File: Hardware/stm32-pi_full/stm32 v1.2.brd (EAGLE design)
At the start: 131.4 x 105.8 mm, 288 parts, among them J1 JUMPER-SMT_2_NC_TRACE_NO-SILK, Q1 PNP, Q2 NPN, Q3 NPN, U1 ESP32-WROOM-32D

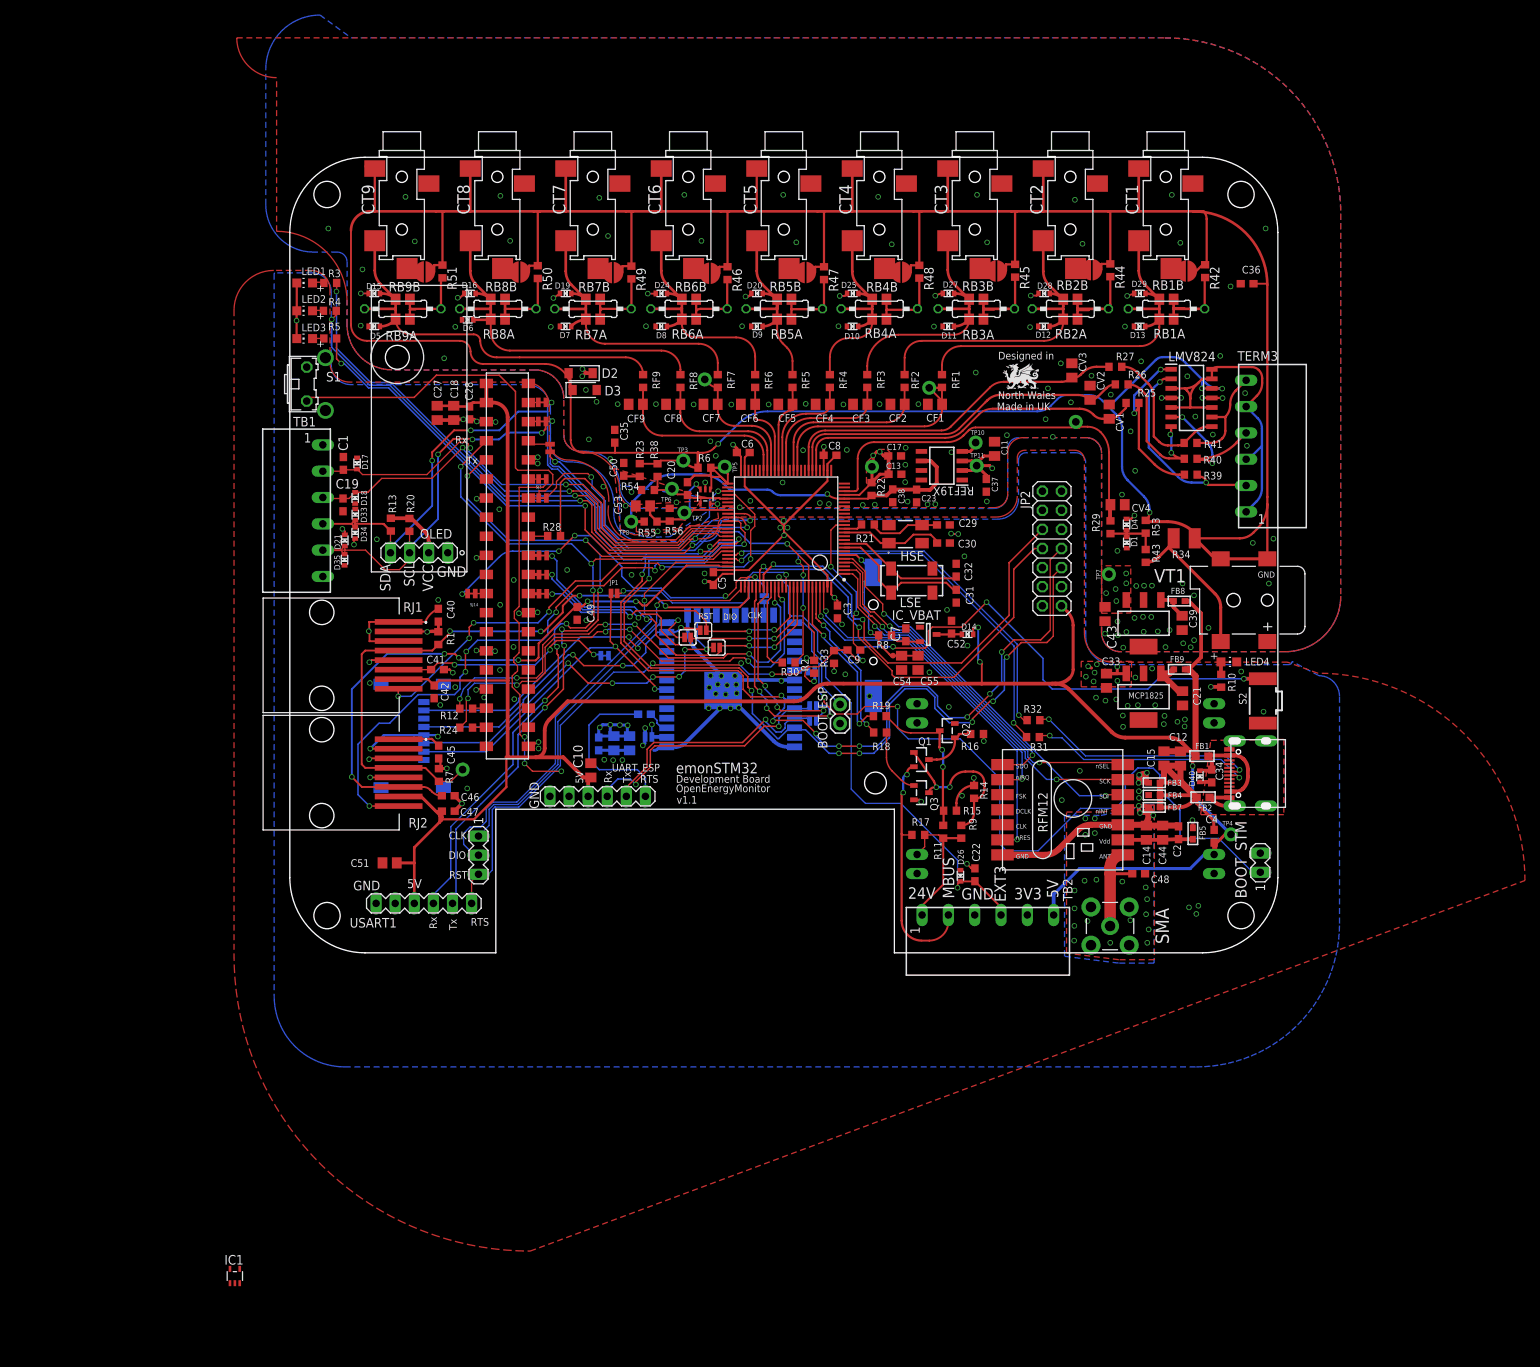
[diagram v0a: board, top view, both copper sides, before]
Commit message: modified:   Hardware/stm32-pi_full/stm32 v1.2.brd 	modified:   Hardware/stm32-pi_full/stm32 v1.2.sch 	modified:   Software/Sombrero_VE_Working6/build/Sombrero_VE_Working6.bin
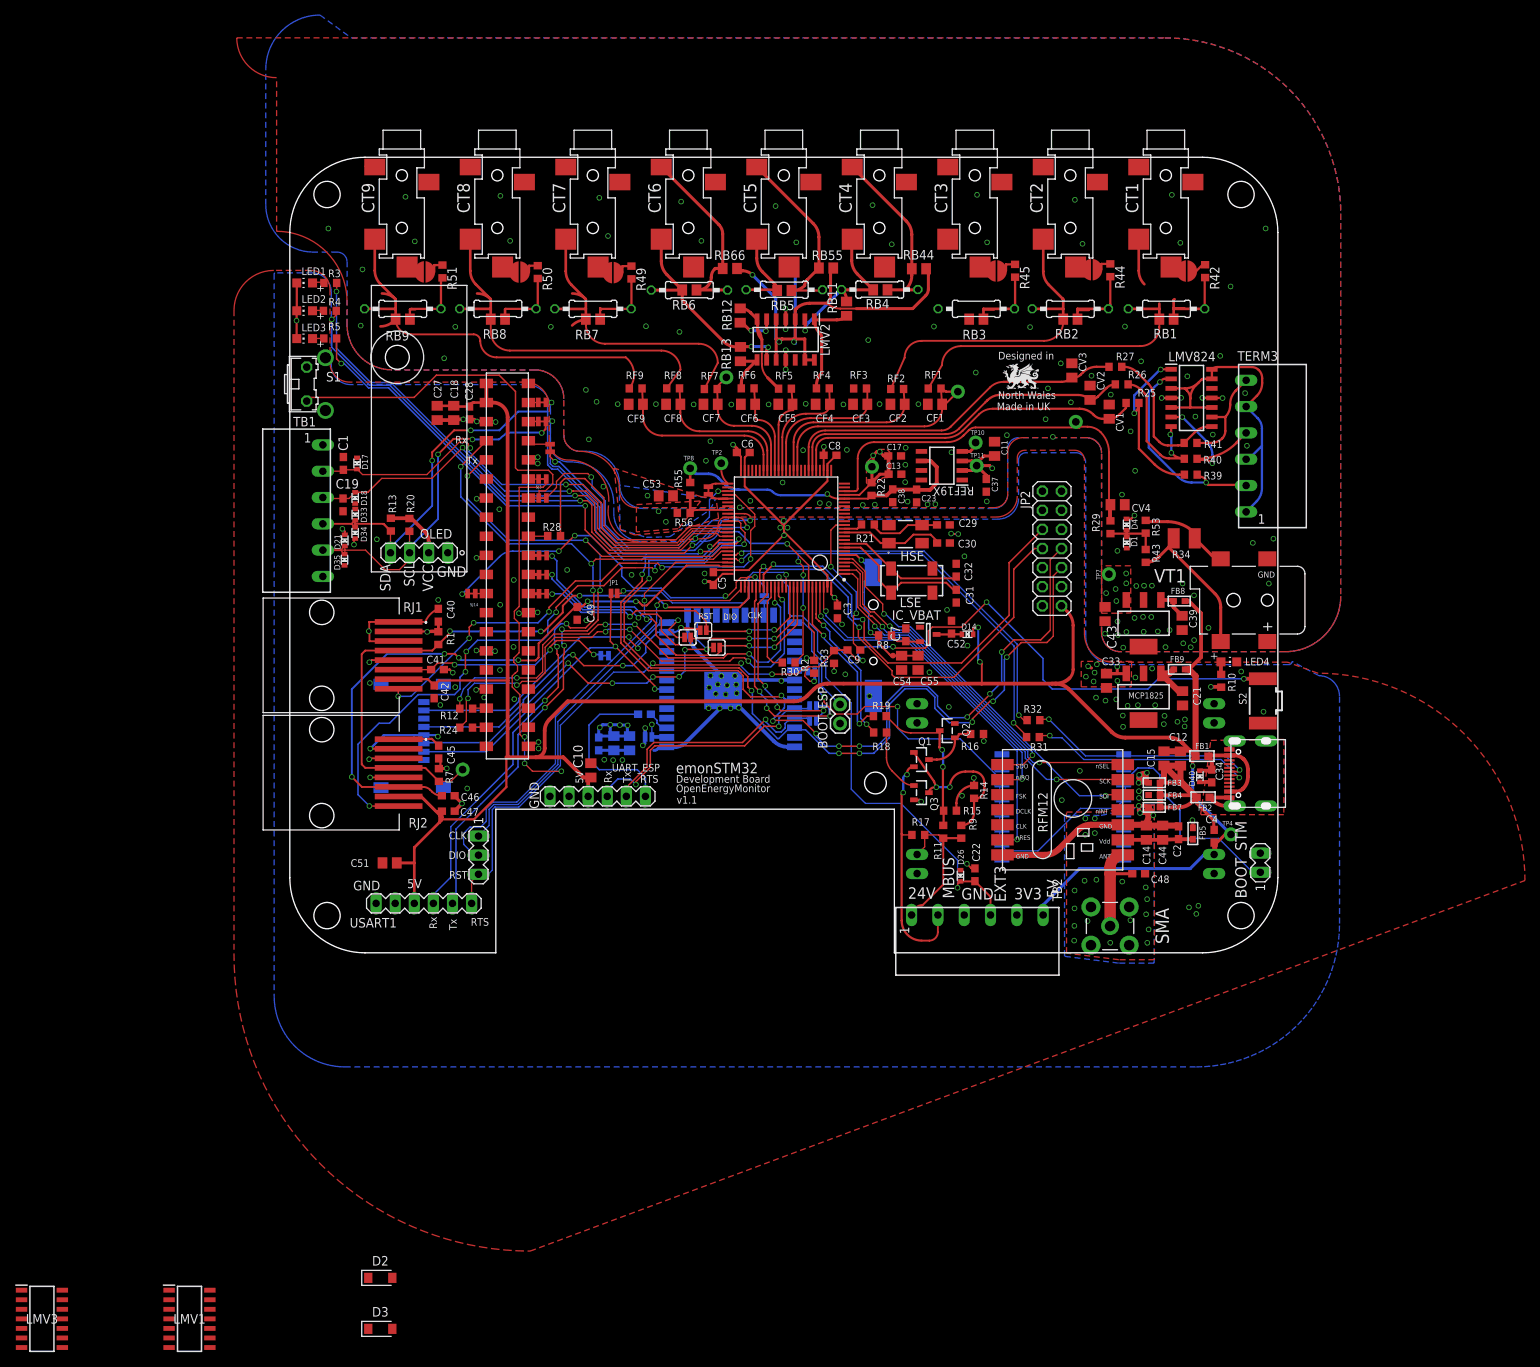
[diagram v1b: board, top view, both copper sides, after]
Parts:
- removed C20: 2.2nF, rcl:C0603
- removed C35, C36: (no value), rcl:C0603
- removed C50: 1uF, rcl:C0603
- removed D10, D11, D12, D13, D15, D16, D19, D20, D24, D25, D27, D28, D29, D5, D6, D7, D8, D9: ESD5Z3.3T1G, microbuilder:SOD-523
- removed IC1, IC2: (no value), analog-devices:SC70-5
- removed JP11, JP13, JP15: JUMPER-SMT_2_NO_NO-SILK_ROUND, SparkFun-Jumpers:SMT-JUMPER_2_NO_NO-SILK_ROUND
- removed R23: 1k, resistor:R0603
- removed R38: 39k, resistor:R0603
- removed R46, R47, R48: 0R, rcl:R0603
- removed R54: 10k, resistor:R0603
- removed R6: 0R, resistor:R0603
- removed RB1B, RB2B, RB3B, RB4B, RB5B, RB6B, RB7B, RB8B, RB9B: (no value), rcl:R0805
- removed RB4A, RB5A, RB6A: 6R8, rcl:R0805
- removed TP3, TP5, TP6: TEST-POINTPOGO_PTH, SparkFun-Connectors:1X01_NO_SILK
- added LMV1, LMV2, LMV3: LMV824IDG4, LMV824IDG4:SOIC127P600X175-14N
- added RB11, RB12, RB13: 510R, rcl:R0805
- added RB4, RB5, RB6: 6R8, rcl:R0805
- added RB44, RB55, RB66: 680R, rcl:R0805
- added SJ1: JUMPER-SMT_2_NC_TRACE_NO-SILK, SparkFun-Jumpers:SMT-JUMPER_2_NC_TRACE_NO-SILK
- added U2: RFM69HCW/RFM95W, microbuilder:RFMHCW_SMT
- R55: value 91k -> 10k
- moved D3 127.8 mm to (12.0, -50.0)
- moved D2 123.2 mm to (12.0, -43.2), turned to 0 degrees
- moved TP8 10.6 mm to (53.2, 64.4)
- moved TP2 8.19 mm to (57.4, 65.1)
- moved R55 6.84 mm to (53.3, 61.7), turned to 90 degrees
- moved TP18 3.84 mm to (88.8, 74.6)
- moved C53 3.33 mm to (50.0, 60.8)
- moved TP19 2.88 mm to (58.1, 76.5)
- moved RB4_ 2.57 mm to (78.4, 88.2)
- moved RB5_ 2.54 mm to (65.8, 88.2)
- moved RB6_ 2.49 mm to (53.1, 88.1)
- moved R56 1.88 mm to (52.4, 58.5), turned to 0 degrees
- moved RF2 1.45 mm to (80.8, 75.0), turned to 0 degrees
- moved RF5 1.43 mm to (65.9, 75.0), turned to 0 degrees
- moved RF7 1.42 mm to (56.0, 75.0), turned to 0 degrees
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- renumbered RB1A to RB1, RB2A to RB2, RB3A to RB3, RB7A to RB7, RB8A to RB8, RB9A to RB9
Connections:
- net CT4 renamed CT4_ADC
- net CT5 renamed CT5_ADC
- net CT6 renamed CT6_ADC
- removed net N$25: R46.2, RB6A.2, RB6B.2, RB6_.2
- new net BIAS1: D2.2, D3.1
- new net BIAS456: LMV2.10, LMV2.13, LMV2.14, LMV2.3, LMV2.5, RB44.2, RB55.2, RB66.2
- new net CT4_OUT: LMV2.1, RB11.1, RF4.1
- new net CT5_OUT: LMV2.7, RB12.1, RF5.1
- new net CT6_OUT: LMV2.8, RB13.2, RF6.1
- new net N$12: CT5.P$3
- new net N$38: CT4.P$3
- new net N$40: CT6.P$1, RB6.2, RB66.1, RB6_.2
- net +3V3ANA: now also LMV1.4, LMV2.4, LMV3.4; no longer D15.K, D16.K, D19.K, D20.K, D24.K, D25.K, D27.K, D28.K, D29.K, IC2.5
- net AGND: now also LMV1.11, LMV2.11, LMV3.11; no longer C35.2, C36.2, C50.2, D10.A, D11.A, D12.A, D13.A, D5.A, D6.A, D7.A, D8.A, D9.A, IC2.2, R54.2
- net BIAS: now also LMV2.12; no longer C35.1, C36.1, CT4.P$1, CT5.P$1, CT6.P$1, D2.2, D3.1, JP11.1, JP13.1, JP15.1, R23.2, R38.1, R46.1, R47.1, R48.1, R6.2, TP3.1
- net CT_IN1: no longer D13.K, D29.A, RB1B.1
- net CT_IN2: no longer D12.K, D28.A, RB2B.1
- net CT_IN3: no longer D11.K, D27.A, RB3B.1
- net CT_IN4: now also LMV2.2, RB11.2, RB4.1; no longer D10.K, D25.A, RB4A.1, RB4B.1, RF4.1
- net CT_IN5: now also LMV2.6, RB12.2, RB5.1; no longer D20.A, D9.K, RB5A.1, RB5B.1, RF5.1
- net CT_IN6: now also LMV2.9, RB13.1, RB6.1; no longer D24.A, D8.K, RB6A.1, RB6B.1, RF6.1
- net CT_IN7: no longer D19.A, D7.K, RB7B.1
- net CT_IN8: no longer D16.A, D6.K, RB8B.1
- net CT_IN9: no longer D15.A, D5.K, RB9B.1
- net DGND: now also U2.16P, U2.2P, U2.9P
- net N$10: no longer JP13.2
- net N$2: no longer JP11.2
- net N$20: no longer JP15.2
- net N$24: now also CT6.P$3; no longer R47.2, RB5A.2, RB5B.2, RB5_.2
- net N$26: no longer RB1B.2
- net N$27: no longer RB2B.2
- net N$29: no longer RB8B.2
- net N$34: no longer RB9B.2
- net N$35: now also CT4.P$1, RB4.2, RB44.1; no longer R48.2, RB4A.2, RB4B.2
- net N$36: no longer RB7B.2
- net N$37: no longer RB3B.2
- net N$7: now also CT5.P$1, RB5.2, RB55.1, RB5_.2; no longer C50.1, R23.1
- net OPAMP_INVERT-: now also SJ1.1; no longer C20.1, IC2.4, R38.2, R54.1, TP6.1
- net OPAMP_NON-INVERT+: no longer IC2.3, TP2.1
- net OPAMP_OUT: now also SJ1.2, TP2.1; no longer C20.2, IC2.1, R6.1, TP5.1
- net VDD: now also U2.5P
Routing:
- net BIAS: track 525.0 -> 26.7 mm, vias 4 -> 0
- net BIAS456: track 0.00 -> 67.5 mm, vias 0 -> 3
- net +3V3ANA: track 73.2 -> 35.3 mm, vias 23 -> 13
- net CT_IN3: track 37.3 -> 0.00 mm
- net N$40: track 0.00 -> 26.0 mm
- net N$7: track 2.18 -> 25.9 mm
- net CT5_OUT: track 0.00 -> 15.7 mm
- net CT4_OUT: track 0.00 -> 13.9 mm
- net N$35: track 11.1 -> 23.9 mm
- net OPAMP_OUT: track 17.4 -> 5.57 mm
- net VREF+: track 53.1 -> 41.5 mm
- net CT_IN5: track 29.6 -> 18.3 mm, vias 0 -> 2
- net N$25: track 11.2 -> 0.00 mm
- net OPAMP_NON-INVERT+: track 18.4 -> 7.42 mm, vias 1 -> 0
- net N$24: track 10.9 -> 0.00 mm
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
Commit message: update
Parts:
- RB1, RB2, RB3, RB4, RB5, RB6, RB7, RB8, RB9: value 6R8 -> 6R81
- RB11, RB12, RB13: value 510R -> 510R 0.1%
- RB44, RB55, RB66: value 680R -> 680R | 681R 0.1%
